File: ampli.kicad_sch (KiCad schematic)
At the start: 51 parts, among them J2 Conn_01x02, J3 Conn_01x03, Q1 2N2907, Q10 TIP32, Q11 BD138, Q12 TIP31, Q13 2N2222, Q2 2N2907, Q3 2N2907, Q4 2N2222, Q5 2N2222, Q6 2N2907, Q7 2N2907, Q8 BD139, Q9 BD139, U1 Relay_1CT, U2 Jack_Mono

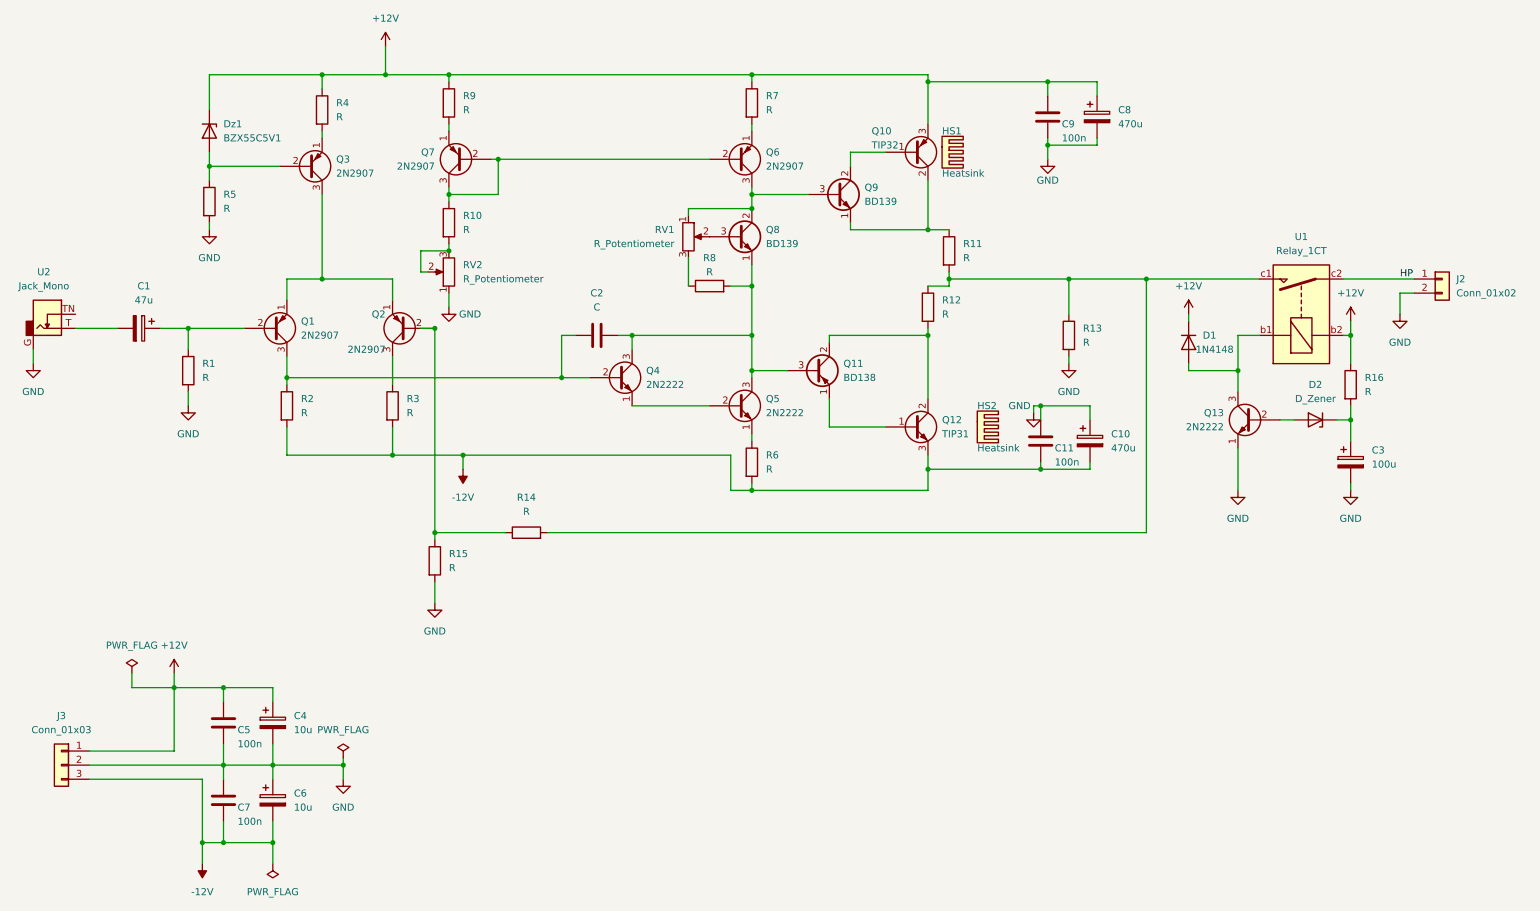
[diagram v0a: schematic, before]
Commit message: .
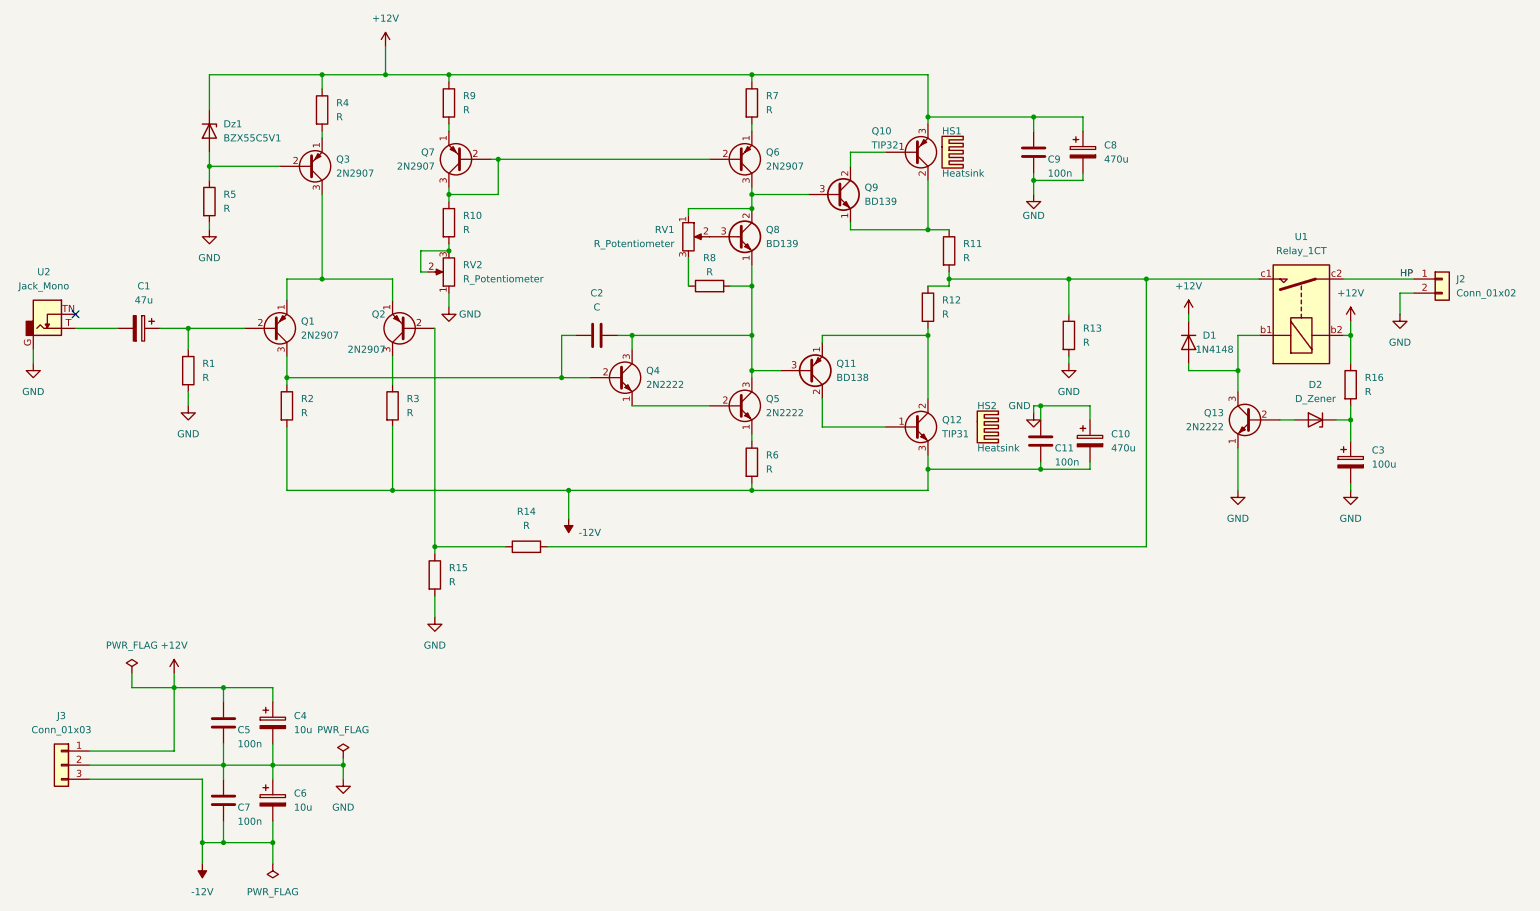
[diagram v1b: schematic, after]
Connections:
- net at Q12.2 (C), R12.2: now also Q11.1 (E); no longer Q11.2 (C)
- net at Q12.1 (B): now also Q11.2 (C); no longer Q11.1 (E)
- no-connect marks 0 -> 1
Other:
- moved on the sheet: C8, C9, Q11, R14, R15

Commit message: .
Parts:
- C1, C4, C6: footprint Capacitor_THT:CP_Radial_D8.0mm_P5.00mm -> CmpAmpliAudioTR:CP_Radial_D8.0mm_P5.00mm
- C10, C3, C8: footprint Capacitor_THT:CP_Radial_D12.5mm_P5.00mm -> CmpAmpliAudioTR:CP_Radial_D12.5mm_P5.00mm
- C11, C2, C5, C7, C9: footprint Capacitor_THT:C_Rect_L7.2mm_W3.5mm_P5.00mm_FKS2_FKP2_MKS2_MKP2 -> CmpAmpliAudioTR:C_Rect_L7.2mm_W3.5mm_P5.00mm_FKS2_FKP2_MKS2_MKP2
- D1: footprint Diode_THT:D_DO-35_SOD27_P7.62mm_Horizontal -> CmpAmpliAudioTR:D_DO-35_SOD27_P10.16mm_Horizontal
- D2, Dz1: footprint Diode_THT:D_DO-35_SOD27_P10.16mm_Horizontal -> CmpAmpliAudioTR:D_DO-35_SOD27_P10.16mm_Horizontal
- HS1, HS2: footprint Heatsink:Heatsink_Fischer_SK104-STC-STIC_35x13mm_2xDrill2.5mm -> CmpAmpliAudioTR:Heatsink_Fischer_SK104-STC-STIC_35x13mm_2xDrill2.5mm
- J2: footprint Connector_Phoenix_MSTB:PhoenixContact_MSTBVA_2,5_2-G-5,08_1x02_P5.08mm_Vertical -> CmpAmpliAudioTR:PhoenixContact_MSTBVA_2,5_2-G-5,08_1x02_P5.08mm_Vertical
- J3: footprint Connector_Phoenix_MSTB:PhoenixContact_MSTBVA_2,5_3-G-5,08_1x03_P5.08mm_Vertical -> CmpAmpliAudioTR:PhoenixContact_MSTBVA_2,5_3-G-5,08_1x03_P5.08mm_Vertical
- Q1, Q13, Q2, Q3, Q4, Q5, Q6, Q7: footprint Package_TO_SOT_THT:TO-18-3 -> CmpAmpliAudioTR:TO-18-3
- Q10, Q12: footprint Package_TO_SOT_THT:TO-220-3_Vertical -> CmpAmpliAudioTR:TO-220-3_Vertical
- Q11, Q8, Q9: footprint Package_TO_SOT_THT:TO-126-3_Vertical -> CmpAmpliAudioTR:TO-126-3_Vertical
- R1, R10, R13, R14, R15, R16, R2, R3, R4, R5, R6, R7, R8, R9: footprint Resistor_THT:R_Axial_DIN0207_L6.3mm_D2.5mm_P10.16mm_Horizontal -> CmpAmpliAudioTR:R_Axial_DIN0207_L6.3mm_D2.5mm_P10.16mm_Horizontal
- R11, R12: footprint R_Axial_DIN0516_L15.5mm_D5.0mm_P20.32mm_Horizontal -> CmpAmpliAudioTR:R_Axial_DIN0516_L15.5mm_D5.0mm_P20.32mm_Horizontal
- RV1, RV2: footprint Potentiometer_THT:Potentiometer_Bourns_3296W_Vertical -> CmpAmpliAudioTR:Potentiometer_Bourns_3296W_Vertical
